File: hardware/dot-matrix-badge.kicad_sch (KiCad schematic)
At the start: 16 parts, among them J1 AVR-UPDI-6, J2 Qwiic/Stemma QT, J3 Test Pads, SW1 SW_SPST, SW2 SW_Push, SW3 SW_Push, U1 HCMS-291X, U2 ATtiny1604-SS

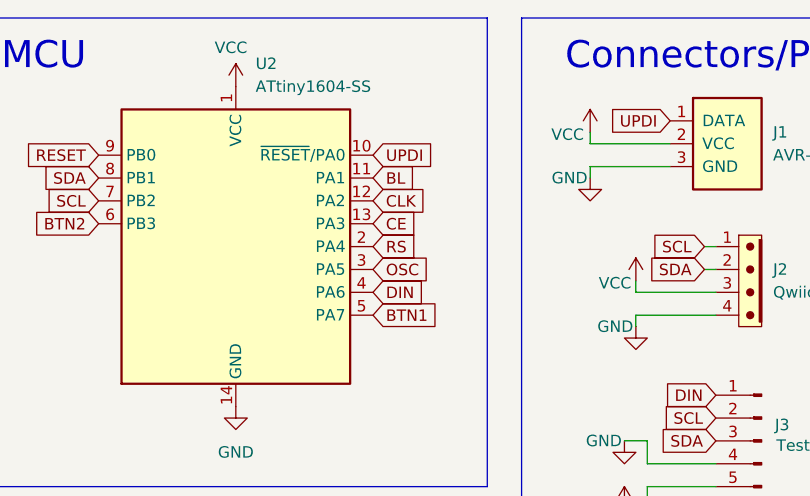
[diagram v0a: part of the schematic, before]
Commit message: done with cleanup, making things pretty
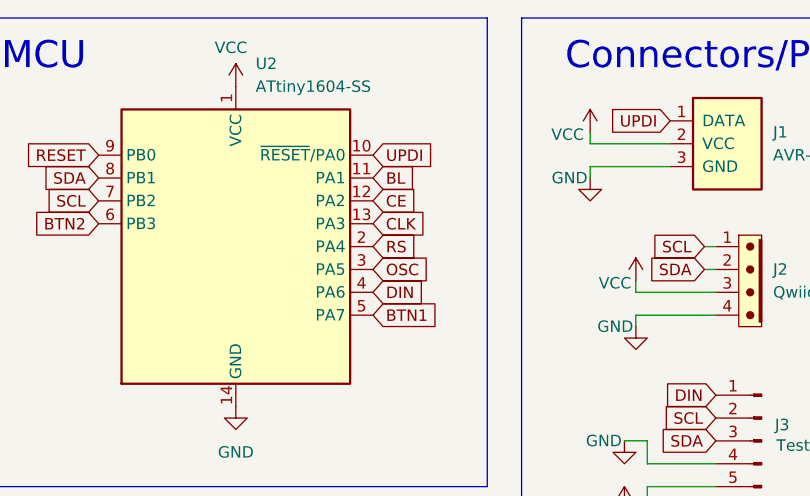
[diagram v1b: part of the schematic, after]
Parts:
- BT1: footprint Battery:BatteryHolder_Keystone_3034_1x20mm -> DotMatrixBadge:BatteryHolder_Keystone_3034_1x20mm
- D1: footprint LED_SMD:LED_0603_1608Metric -> DotMatrixBadge:LED_0603_1608Metric
- R1: footprint Resistor_SMD:R_0603_1608Metric -> DotMatrixBadge:R_0603_1608Metric
- SW1: footprint Button_Switch_SMD:SW_SPDT_PCM12 -> DotMatrixBadge:SW_SPDT_PCM12
- U2: footprint Package_SO:SOIC-14_3.9x8.7mm_P1.27mm -> DotMatrixBadge:SOIC-14_3.9x8.7mm_P1.27mm
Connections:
- net CE: now also U2.12 (PA2); no longer U2.13 (PA3)
- net CLK: now also U2.13 (PA3); no longer U2.12 (PA2)
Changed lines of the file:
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@@
+	(global_label "CE"
+		(shape input)
+		(at 119.38 35.56 0)
+		(fields_autoplaced yes)
+		(effects
+			(font
+				(size 1.27 1.27)
+			)
+			(justify left)
+		)
+		(property "Intersheetrefs" "${INTERSHEET_REFS}"
+			(at 124.7842 35.56 0)
+			(effects
+				(font
+					(size 1.27 1.27)
+				)
+				(justify left)
+				(hide yes)
+			)
+		)
+	)
 	(global_label "CE"
 		(shape input)
@@
 		)
 	)
-	(global_label "CLK"
+	(global_label "OSC"
 		(shape input)
-		(at 119.38 35.56 0)
+		(at 119.38 43.18 0)
 		(fields_autoplaced yes)
 		(effects
@@
 		)
 		(property "Intersheetrefs" "${INTERSHEET_REFS}"
-			(at 125.9333 35.56 0)
-			(effects
-				(font
-					(size 1.27 1.27)
-				)
-				(justify left)
-				(hide yes)
-			)
-		)
-	)
-	(global_label "OSC"
+			(at 126.1752 43.18 0)
+			(effects
+				(font
+					(size 1.27 1.27)
+				)
+				(justify left)
+				(hide yes)
+			)
+		)
+	)
+	(global_label "CLK"
 		(shape input)
-		(at 119.38 43.18 0)
+		(at 119.38 38.1 0)
 		(fields_autoplaced yes)
 		(effects
@@
 		)
 		(property "Intersheetrefs" "${INTERSHEET_REFS}"
-			(at 126.1752 43.18 0)
+			(at 125.9333 38.1 0)
 			(effects
 				(font
@@
 		)
 	)
-	(global_label "CE"
+	(global_label "BL"
 		(shape input)
-		(at 119.38 38.1 0)
+		(at 119.38 33.02 0)
 		(fields_autoplaced yes)
 		(effects
@@
 		)
 		(property "Intersheetrefs" "${INTERSHEET_REFS}"
-			(at 124.7842 38.1 0)
-			(effects
-				(font
-					(size 1.27 1.27)
-				)
-				(justify left)
-				(hide yes)
-			)
-		)
-	)
-	(global_label "BL"
+			(at 124.6633 33.02 0)
+			(effects
+				(font
+					(size 1.27 1.27)
+				)
+				(justify left)
+				(hide yes)
+			)
+		)
+	)
+	(global_label "SCL"
 		(shape input)
-		(at 119.38 33.02 0)
+		(at 156.21 40.64 180)
 		(fields_autoplaced yes)
 		(effects
@@
 				(size 1.27 1.27)
 			)
-			(justify left)
+			(justify right)
 		)
 		(property "Intersheetrefs" "${INTERSHEET_REFS}"
-			(at 124.6633 33.02 0)
-			(effects
-				(font
-					(size 1.27 1.27)
-				)
-				(justify left)
+			(at 149.7172 40.64 0)
+			(effects
+				(font
+					(size 1.27 1.27)
+				)
+				(justify right)
 				(hide yes)
 			)
@@
 	(global_label "SCL"
 		(shape input)
-		(at 156.21 40.64 180)
+		(at 157.48 59.69 180)
 		(fields_autoplaced yes)
 		(effects
@@
 		)
 		(property "Intersheetrefs" "${INTERSHEET_REFS}"
-			(at 149.7172 40.64 0)
+			(at 150.9872 59.69 0)
 			(effects
 				(font
@@
 		)
 	)
-	(global_label "SCL"
+	(global_label "DOUT"
 		(shape input)
-		(at 157.48 59.69 180)
+		(at 30.48 60.96 180)
 		(fields_autoplaced yes)
 		(effects
@@
 		)
 		(property "Intersheetrefs" "${INTERSHEET_REFS}"
-			(at 150.9872 59.69 0)
+			(at 22.5962 60.96 0)
 			(effects
 				(font
@@
 		)
 	)
-	(global_label "DOUT"
+	(global_label "SDA"
 		(shape input)
-		(at 30.48 60.96 180)
+		(at 88.9 33.02 180)
 		(fields_autoplaced yes)
 		(effects
@@
 		)
 		(property "Intersheetrefs" "${INTERSHEET_REFS}"
-			(at 22.5962 60.96 0)
+			(at 82.3467 33.02 0)
 			(effects
 				(font
@@
 		)
 	)
-	(global_label "SDA"
+	(global_label "UPDI"
 		(shape input)
-		(at 88.9 33.02 180)
+		(at 152.4 26.67 180)
 		(fields_autoplaced yes)
 		(effects
@@
 		)
 		(property "Intersheetrefs" "${INTERSHEET_REFS}"
-			(at 82.3467 33.02 0)
+			(at 144.9395 26.67 0)
 			(effects
 				(font
@@
 		)
 	)
-	(global_label "UPDI"
+	(global_label "SDA"
 		(shape input)
-		(at 152.4 26.67 180)
+		(at 157.48 62.23 180)
 		(fields_autoplaced yes)
 		(effects
@@
 		)
 		(property "Intersheetrefs" "${INTERSHEET_REFS}"
-			(at 144.9395 26.67 0)
-			(effects
-				(font
-					(size 1.27 1.27)
-				)
-				(justify right)
-				(hide yes)
-			)
-		)
-	)
-	(global_label "SDA"
-		(shape input)
-		(at 157.48 62.23 180)
-		(fields_autoplaced yes)
-		(effects
-			(font
-				(size 1.27 1.27)
-			)
-			(justify right)
-		)
-		(property "Intersheetrefs" "${INTERSHEET_REFS}"
 			(at 150.9267 62.23 0)
 			(effects
@@
 			)
 		)
-		(property "Footprint" "LED_SMD:LED_0603_1608Metric"
+		(property "Footprint" "DotMatrixBadge:LED_0603_1608Metric"
 			(at 118.11 110.49 0)
 			(effects
@@
 			)
 		)
-		(property "Footprint" "Button_Switch_SMD:SW_SPDT_PCM12"
+		(property "Footprint" "DotMatrixBadge:SW_SPDT_PCM12"
 			(at 48.26 97.79 0)
 			(effects
@@
 			)
 		)
-		(property "Footprint" "Resistor_SMD:R_0603_1608Metric"
+		(property "Footprint" "DotMatrixBadge:R_0603_1608Metric"
 			(at 109.601 106.172 0)
 			(effects
@@
 			)
 		)
-		(property "Footprint" "Battery:BatteryHolder_Keystone_3034_1x20mm"
+		(property "Footprint" "DotMatrixBadge:BatteryHolder_Keystone_3034_1x20mm"
 			(at 48.26 106.426 90)
 			(effects
@@
 			)
 		)
-		(property "Footprint" "Package_SO:SOIC-14_3.9x8.7mm_P1.27mm"
+		(property "Footprint" "DotMatrixBadge:SOIC-14_3.9x8.7mm_P1.27mm"
 			(at 104.14 40.64 0)
 			(effects
